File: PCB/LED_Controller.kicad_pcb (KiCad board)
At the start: 2 copper layers, 48.3 x 58.4 mm, 45 parts, among them J1 Conn_01x04_Female, J2 Conn_01x06_Female, J3 Conn_01x06_Female, J4 Add. LED Strip, J5 Add. LED Strip, J7 Conn_01x02, Q1 MMBF170, Q10 BC817, Q2 MMBF170, Q3 MMBF170, Q4 MMBF170, Q9 BC817, SW1 SW_Push, SW2 SW_Push, U1 ESP32-WROOM-32, U2 NCP1117-5.0_SOT223, U3 NCP1117-3.3_SOT223

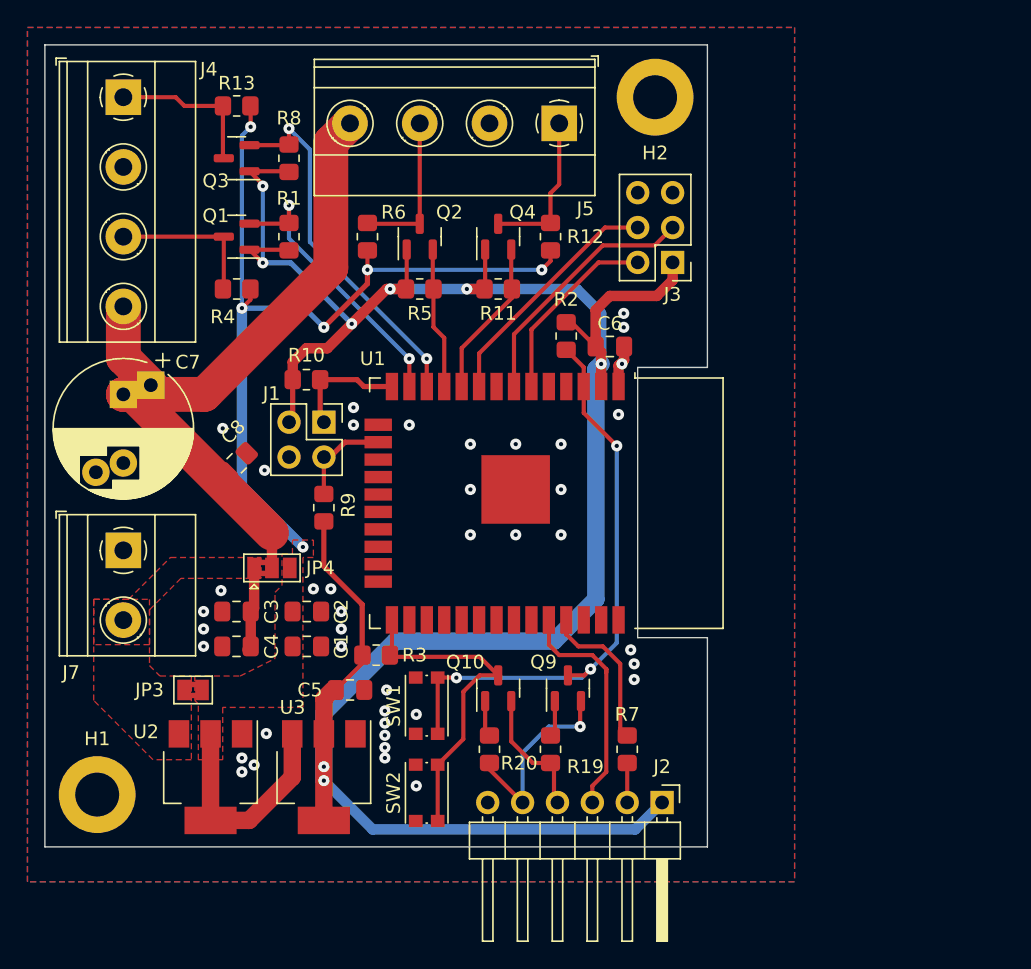
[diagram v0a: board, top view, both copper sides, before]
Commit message: Rev 2.0 local push
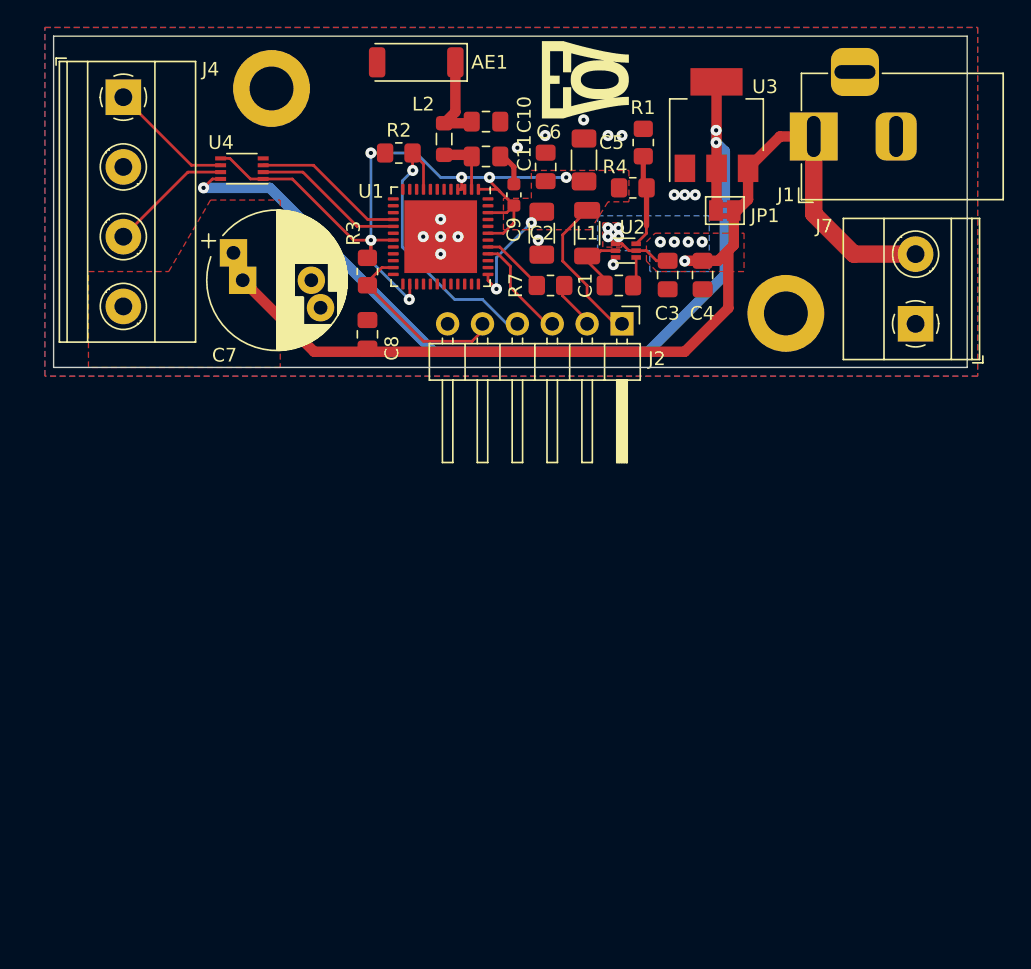
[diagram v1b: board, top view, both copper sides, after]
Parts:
- removed J3: Conn_01x06_Female, Connector_PinHeader_2.54mm:PinHeader_2x03_P2.54mm_Vertical
- removed J5: Add. LED Strip, TerminalBlock_Phoenix:TerminalBlock_Phoenix_MKDS-1,5-4-5.08_1x04_P5.08mm_Horizontal
- removed JP3: Jumper_2_Bridged, Jumper:SolderJumper-2_P1.3mm_Bridged2Bar_Pad1.0x1.5mm
- removed JP4: Jumper_3_Bridged12, Jumper:SolderJumper-3_P1.3mm_Bridged2Bar12_Pad1.0x1.5mm
- removed Q1, Q2, Q3, Q4: MMBF170, Package_TO_SOT_SMD:SOT-23
- removed Q10, Q9: BC817, Package_TO_SOT_SMD:SOT-23
- removed R10, R11, R12, R13, R19, R20, R5, R6, R8, R9: 10k, Resistor_SMD:R_0805_2012Metric_Pad1.20x1.40mm_HandSolder
- removed SW1, SW2: SW_Push, Button_Switch_SMD:SW_Push_1P1T_NO_CK_KMR2
- added AE1: Antenna_Chip, RF_Antenna:Johanson_2450AT43F0100, F.Cu at (156.6, 55.9)
- added C10: C, Capacitor_SMD:C_0805_2012Metric_Pad1.18x1.45mm_HandSolder, F.Cu at (161.7, 62.7)
- added C11: C, Capacitor_SMD:C_0805_2012Metric_Pad1.18x1.45mm_HandSolder, F.Cu at (161.7, 60.2)
- added C9: 0.1u, Capacitor_SMD:C_0603_1608Metric, F.Cu at (163.7, 65.5)
- added G***: LOGO, LOGO, F.Cu at (168.9, 57.1)
- added JP1: Jumper_2_Bridged, Jumper:SolderJumper-2_P1.3mm_Bridged2Bar_Pad1.0x1.5mm, F.Cu at (179.1, 66.7)
- added L1: 3.3uH, Inductor_SMD:L_1206_3216Metric_Pad1.22x1.90mm_HandSolder, F.Cu at (169.0, 68.3)
- added L2: L, Inductor_SMD:L_0805_2012Metric_Pad1.05x1.20mm_HandSolder, F.Cu at (158.6, 61.5)
- added U4: 74LVCH2T45DC, Package_SO:VSSOP-8_2.3x2mm_P0.5mm, F.Cu at (143.9, 63.6)
- C1: value 10uF -> 0.1uF
- C2: value 0.1uF -> 22uF; footprint Capacitor_SMD:C_0805_2012Metric_Pad1.18x1.45mm_HandSolder -> Capacitor_SMD:C_1206_3216Metric_Pad1.33x1.80mm_HandSolder
- C5: footprint Capacitor_SMD:C_0805_2012Metric_Pad1.18x1.45mm_HandSolder -> Capacitor_SMD:C_1206_3216Metric_Pad1.33x1.80mm_HandSolder
- J1: value Conn_01x04_Female -> Barrel_Jack; footprint Connector_PinHeader_2.54mm:PinHeader_2x02_P2.54mm_Vertical -> Connector_BarrelJack:BarrelJack_Horizontal
- R4: value 10k -> 31.6k
- U1: value ESP32-WROOM-32 -> ESP32-PICO-D4; footprint RF_Module:ESP32-WROOM-32 -> Package_DFN_QFN:QFN-48-1EP_7x7mm_P0.5mm_EP5.3x5.3mm
- U2: value NCP1117-5.0_SOT223 -> AP62200; footprint Package_TO_SOT_SMD:SOT-223-3_TabPin2 -> Package_TO_SOT_SMD:SOT-563
- U3: value NCP1117-3.3_SOT223 -> NCP1117-5.0_SOT223
- moved H1 61.2 mm to (183.5, 74.2)
- moved J7 60.0 mm to (193.0, 74.9), turned to 90 degrees
- moved U3 55.4 mm to (178.5, 60.5), turned to 90 degrees
- moved U2 48.8 mm to (171.9, 69.6), turned to 0 degrees
- moved C4 43.4 mm to (177.4, 71.4), turned to -90 degrees
- moved C5 42.2 mm to (168.8, 63.0), turned to 90 degrees
- moved J1 41.3 mm to (185.5, 61.3), turned to 180 degrees
- moved C3 39.8 mm to (174.9, 71.4), turned to -90 degrees
- moved G*** 35.1 mm to (181.6, 67.3)
- moved J2 35.0 mm to (171.6, 74.9)
- moved C1 34.8 mm to (171.3, 72.1), turned to 180 degrees
- moved R7 34.2 mm to (166.4, 72.1), turned to 0 degrees
- moved C2 32.4 mm to (165.7, 68.3), turned to -90 degrees
- moved R4 29.8 mm to (172.4, 65.0)
- moved H2 27.9 mm to (146.1, 57.8)
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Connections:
- C1 pad 1: +5V -> Net-(C1-Pad1)
- C1 pad 2: GND -> Net-(C1-Pad2)
- C2 pad 1: +5V -> +3V3
- C7 pad 1: VLED -> VIN
- C8 pad 1: VLED -> VIN
- J1 pad 1: /SCL -> VIN
- J1 pad 2: /SDA -> GND
- J1 pad 3: +3V3 -> (no net)
- J2 pad 2: /TX -> Net-(J2-Pad2)
- J2 pad 4: /PROG_DTR -> /EN
- J2 pad 5: /PROG_RTS -> /GPIO0
- J4 pad 4: VLED -> VIN
- R1 pad 1: +3V3 -> GND
- R1 pad 2: /LED1-DATA_{L} -> Net-(R1-Pad2)
- R4 pad 1: +5V -> Net-(R1-Pad2)
- R4 pad 2: /LED1-DATA_{H} -> +3V3
- R7 pad 1: Net-(R7-Pad1) -> /TX
- R7 pad 2: /TX -> Net-(J2-Pad2)
- U1 pad 1: GND -> +3V3
- U1 pad 10: /LED2-CLK_{L} -> /MIC_WS
- U1 pad 11: /LED2-DATA_{L} -> /MIC_SD
- U1 pad 12: /LED1-CLK_{L} -> unconnected-(U1-Pad12)
- U1 pad 13: /LED1-DATA_{L} -> /MIC_SCK
- U1 pad 14: /SCL -> unconnected-(U1-Pad14)
- U1 pad 15: GND -> unconnected-(U1-Pad15)
- U1 pad 16: /SDA -> /LED1-CLK_{L}
- U1 pad 17: unconnected-(U1-Pad17) -> /LED1-DATA_{L}
- U1 pad 19: unconnected-(U1-Pad19) -> +3V3
- U1 pad 2: +3V3 -> Net-(C10-Pad1)
- U1 pad 23: unconnected-(U1-Pad23) -> /GPIO0
- U1 pad 25: /GPIO0 -> unconnected-(U1-Pad25)
- U1 pad 26: unconnected-(U1-Pad26) -> +3V3
- U1 pad 3: /EN -> +3V3
- U1 pad 34: /RX -> unconnected-(U1-Pad34)
- U1 pad 35: Net-(R7-Pad1) -> unconnected-(U1-Pad35)
- U1 pad 37: unconnected-(U1-Pad37) -> +3V3
- U1 pad 38: GND -> unconnected-(U1-Pad38)
- U1 pad 39: GND -> unconnected-(U1-Pad39)
- U1 pad 4: unconnected-(U1-Pad4) -> +3V3
- U1 pad 6: /MIC_WS -> unconnected-(U1-Pad6)
- U1 pad 7: /MIC_SD -> unconnected-(U1-Pad7)
- U1 pad 9: /MIC_SCK -> /EN
- U2 pad 1: GND -> VIN
- U2 pad 2: +5V -> Net-(C1-Pad2)
- U2 pad 3: VIN -> GND
- U3 pad 2: +3V3 -> +5V
- U3 pad 3: +5V -> VIN
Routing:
- net +3V3: track 177.2 -> 76.8 mm
- net VIN: track 6.17 -> 78.9 mm, vias 0 -> 9
- net VLED: track 54.1 -> 0.00 mm
- net /EN: track 42.9 -> 21.1 mm, vias 3 -> 1
- net /MIC_SD: track 18.6 -> 0.00 mm
- net /MIC_SCK: track 17.8 -> 0.00 mm
- net /LED1-CLK_{L}: track 26.9 -> 11.1 mm, vias 2 -> 0
- net /PROG_RTS: track 14.4 -> 0.00 mm, vias 1 -> 0
- net /MIC_WS: track 13.9 -> 0.00 mm
- net +5V: track 80.4 -> 66.9 mm, vias 6 -> 3
- net /GPIO0: track 24.6 -> 12.9 mm
- net /LED2-CLK_{L}: track 11.5 -> 0.00 mm
- net /LED2-CLK_{H}: track 11.4 -> 0.00 mm
- net Net-(R7-Pad1): track 11.3 -> 0.00 mm
- net /LED2-DATA_{H}: track 11.2 -> 0.00 mm
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- added copper zone on F.Cu, net +3V3
- added copper zone on B.Cu, net VIN
- removed copper zone on F.Cu, net +5V
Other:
- board size 48.3 x 58.4 mm -> 66.5 x 24.1 mm
- board text added: "Rev 2"
- board text removed: "Rev 1"
